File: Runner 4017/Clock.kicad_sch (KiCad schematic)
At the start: 7 parts, among them U801 LM555xN

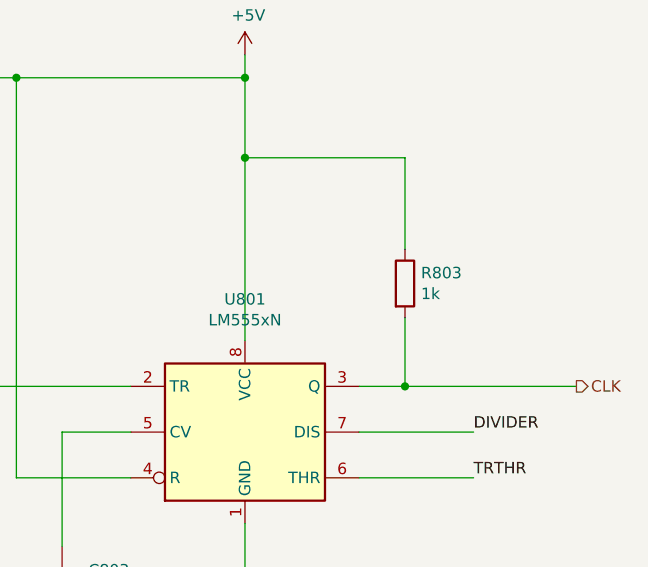
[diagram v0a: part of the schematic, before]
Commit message: Working through things
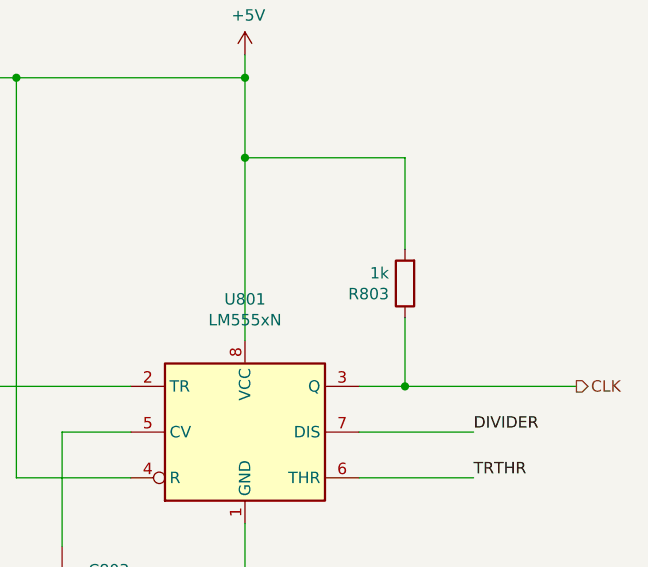
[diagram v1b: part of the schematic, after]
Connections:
- net +5V: now also R803.2; no longer R803.1
- net CLK: now also R803.1; no longer R803.2
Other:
- moved on the sheet: R803
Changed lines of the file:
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@@
     (effects (font (size 1.27 1.27)) (justify left))
   )
-  (symbol (lib_id "Device:R") (at 143.51 77.47 0) (unit 1)
+  (symbol (lib_id "Device:R") (at 143.51 77.47 180) (unit 1)
     (in_bom yes) (on_board yes) (dnp no)
-    (property "Reference" "R803" (at 145.288 76.3016 0)
+    (property "Reference" "R803" (at 141.732 78.6384 0)
       (effects (font (size 1.27 1.27)) (justify left))
     )
-    (property "Value" "1k" (at 145.288 78.613 0)
+    (property "Value" "1k" (at 141.732 76.327 0)
       (effects (font (size 1.27 1.27)) (justify left))
     )
-    (property "Footprint" "Resistor_THT:R_Axial_DIN0207_L6.3mm_D2.5mm_P7.62mm_Horizontal" (at 141.732 77.47 90)
+    (property "Footprint" "Resistor_THT:R_Axial_DIN0207_L6.3mm_D2.5mm_P7.62mm_Horizontal" (at 145.288 77.47 90)
       (effects (font (size 1.27 1.27)) hide)
     )
